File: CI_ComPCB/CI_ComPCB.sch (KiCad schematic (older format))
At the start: 9 parts, among them J101 Conn_01x15_Female, J102 Conn_01x15_Female, U101 ESP32s

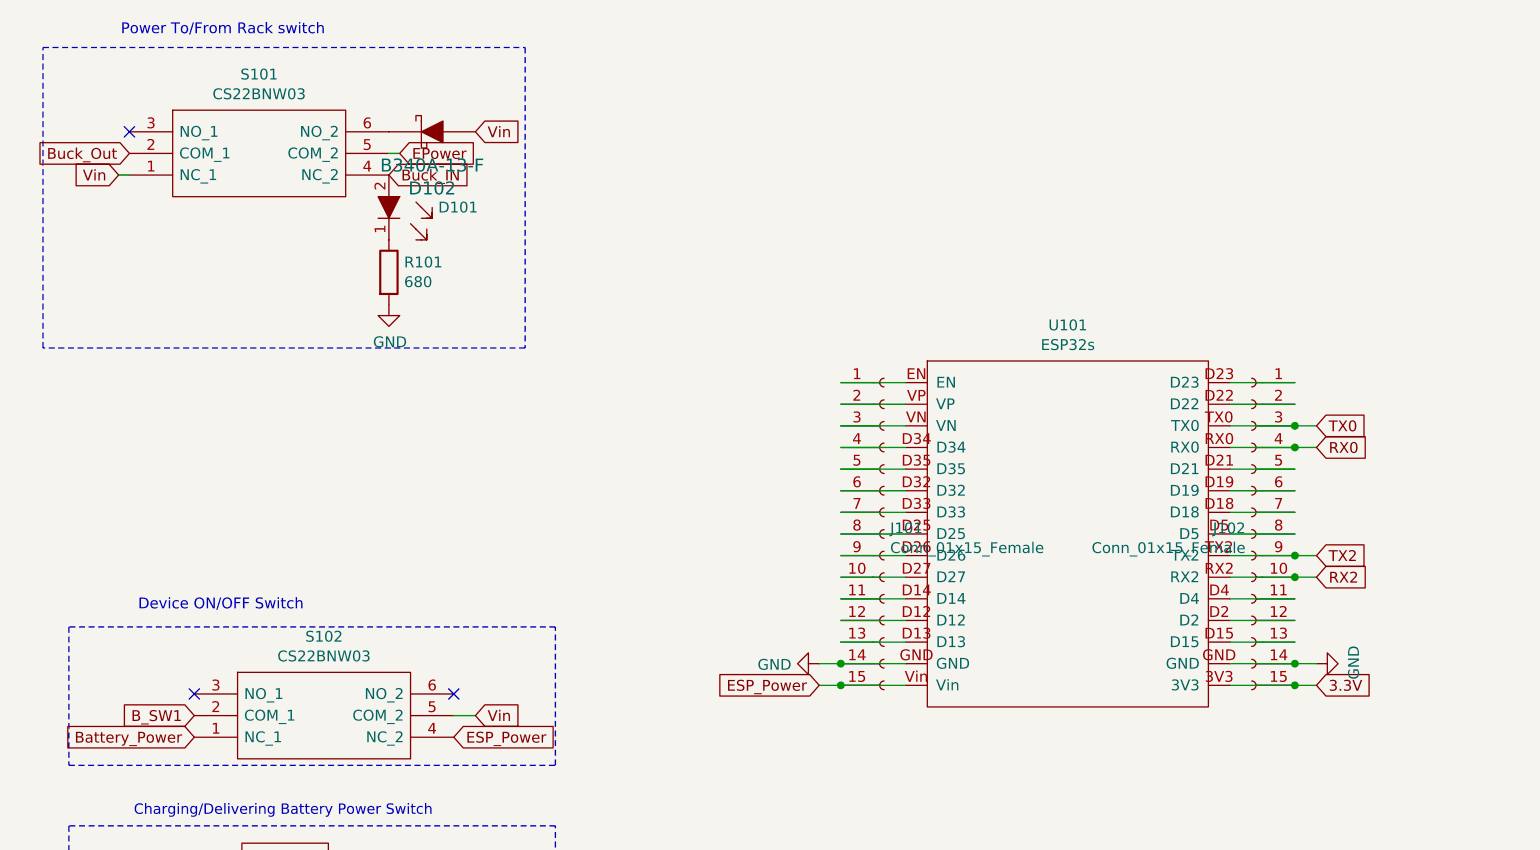
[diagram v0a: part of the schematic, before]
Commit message: V1.1 in progress
Completed Bom and schematic
still need to add routs and PCB layout
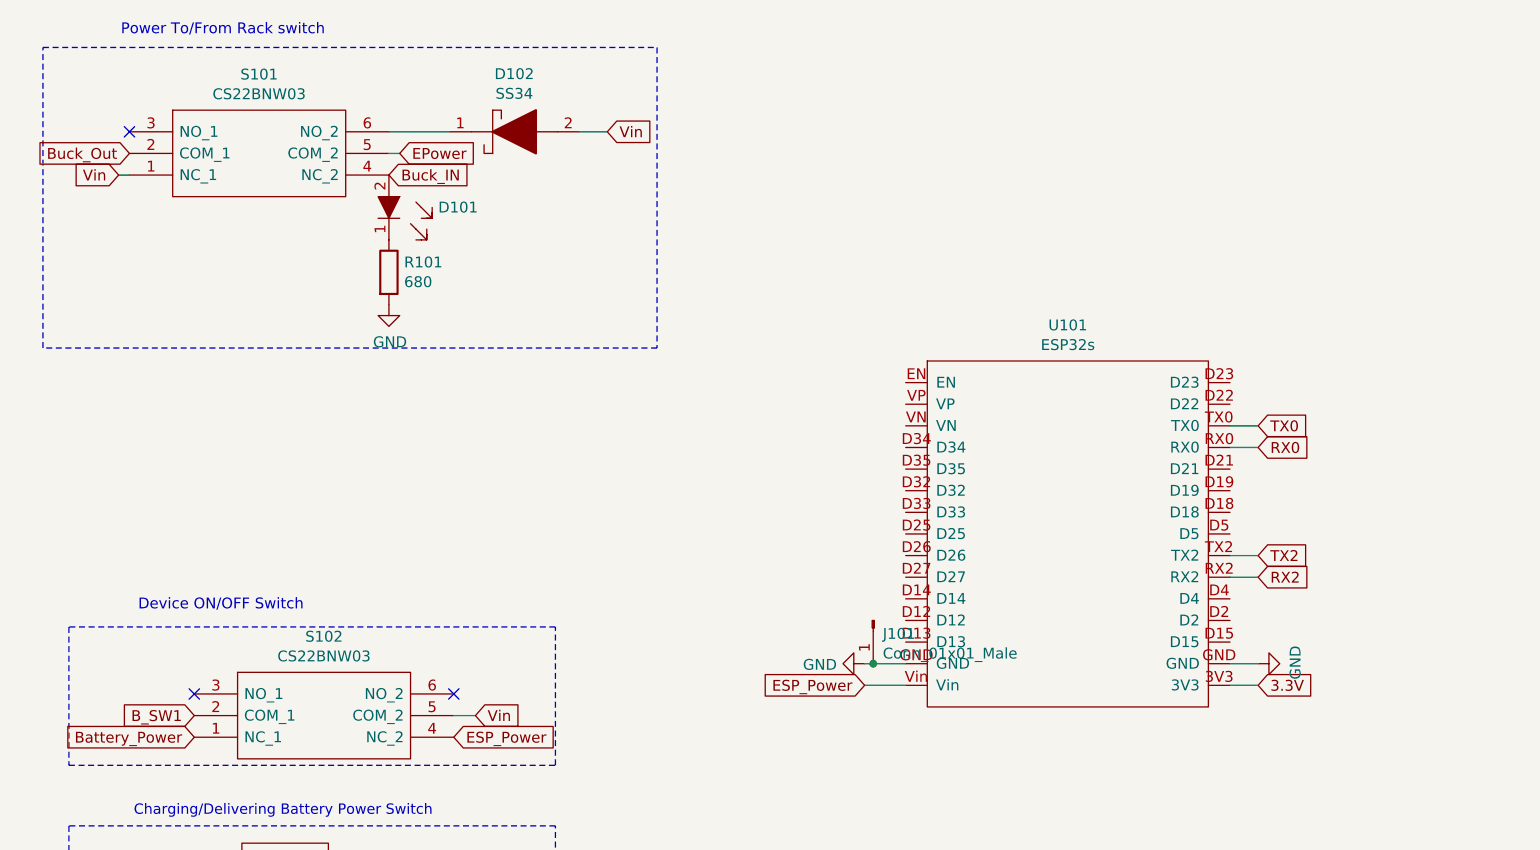
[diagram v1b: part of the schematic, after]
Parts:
- removed D102: B340A-13-F, digikey-footprints:DO-214AC, symbol dk_Diodes-Rectifiers-Single:B340A-13-F
- removed J101, J102: Conn_01x15_Female, Connector_PinSocket_2.54mm:PinSocket_1x15_P2.54mm_Vertical, symbol Connector:Conn_01x15_Female
- added D102: SS34, SamacSys_Parts:DIOM8059X256N, symbol SamacSys_Parts:SS34
- added J101: Conn_01x01_Male, Connector_PinHeader_2.54mm:PinHeader_1x01_P2.54mm_Vertical, symbol Connector:Conn_01x01_Male
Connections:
- net GND: now also J101.1 (Pin_1)
- net Vin: now also D102.2
- net at S101.6 (NO_2): now also D102.1
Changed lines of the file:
@@
 Comment4 ""
 $EndDescr
-Text GLabel 6750 3220 2    50   Input ~ 0
+Text GLabel 6480 3220 2    50   Input ~ 0
 RX0
-Text GLabel 6750 3120 2    50   Input ~ 0
+Text GLabel 6480 3120 2    50   Input ~ 0
 TX0
-Text GLabel 6750 3720 2    50   Input ~ 0
+Text GLabel 6480 3720 2    50   Input ~ 0
 TX2
-Text GLabel 6750 3820 2    50   Input ~ 0
+Text GLabel 6480 3820 2    50   Input ~ 0
 RX2
-Text GLabel 6750 4320 2    50   Input ~ 0
+Text GLabel 6480 4320 2    50   Input ~ 0
 3.3V
 $Comp
@@
 L power:GND #PWR0103
 U 1 1 6128A8B5
-P 6750 4220
-F 0 "#PWR0103" H 6750 3970 50  0001 C CNN
-F 1 "GND" H 6755 4047 50  0000 C CNN
-F 2 "" H 6750 4220 50  0001 C CNN
-F 3 "" H 6750 4220 50  0001 C CNN
-	1    6750 4220
+P 6480 4220
+F 0 "#PWR0103" H 6480 3970 50  0001 C CNN
+F 1 "GND" H 6485 4047 50  0000 C CNN
+F 2 "" H 6480 4220 50  0001 C CNN
+F 3 "" H 6480 4220 50  0001 C CNN
+	1    6480 4220
 	0    -1   -1   0
 $EndComp
@@
 L power:GND #PWR0102
 U 1 1 612B87BD
-P 4450 4220
-F 0 "#PWR0102" H 4450 3970 50  0001 C CNN
-F 1 "GND" V 4455 4092 50  0000 R CNN
-F 2 "" H 4450 4220 50  0001 C CNN
-F 3 "" H 4450 4220 50  0001 C CNN
-	1    4450 4220
+P 4660 4220
+F 0 "#PWR0102" H 4660 3970 50  0001 C CNN
+F 1 "GND" V 4665 4092 50  0000 R CNN
+F 2 "" H 4660 4220 50  0001 C CNN
+F 3 "" H 4660 4220 50  0001 C CNN
+	1    4660 4220
 	0    1    1    0
 $EndComp
@@
 Text Notes 1300 3980 0    50   ~ 0
 Device ON/OFF Switch
-Text GLabel 4450 4320 0    50   Input ~ 0
+Text GLabel 4660 4320 0    50   Input ~ 0
 ESP_Power
 Wire Wire Line
@@
 Text Notes 1220 1320 0    50   ~ 0
 Power To/From Rack switch
-Text GLabel 2860 1760 2    50   Input ~ 0
+Text GLabel 3470 1760 2    50   Input ~ 0
 Vin
 Wire Wire Line
@@
 $EndComp
 Wire Notes Line
-	3090 2760 860  2760
+	3700 2760 860  2760
 Wire Notes Line
 	860  2760 860  1370
 Wire Notes Line
-	860  1370 3090 1370
-Wire Notes Line
-	3090 1370 3090 2760
+	860  1370 3700 1370
+Wire Notes Line
+	3700 1370 3700 2760
 Wire Notes Line
 	980  4690 3230 4690
@@
 Wire Notes Line
 	980  4050 980  4690
-$Comp
-L dk_Diodes-Rectifiers-Single:B340A-13-F D102
-U 1 1 619E1DE9
-P 2660 1760
-F 0 "D102" H 2660 2022 60  0000 C CNN
-F 1 "B340A-13-F" H 2660 1916 60  0000 C CNN
-F 2 "digikey-footprints:DO-214AC" H 2860 1960 60  0001 L CNN
-F 3 "https://www.diodes.com/assets/Datasheets/ds30891.pdf" H 2860 2060 60  0001 L CNN
-F 4 "B340A-FDICT-ND" H 2860 2160 60  0001 L CNN "Digi-Key_PN"
-F 5 "B340A-13-F" H 2860 2260 60  0001 L CNN "MPN"
-F 6 "Discrete Semiconductor Products" H 2860 2360 60  0001 L CNN "Category"
-F 7 "Diodes - Rectifiers - Single" H 2860 2460 60  0001 L CNN "Family"
-F 8 "https://www.diodes.com/assets/Datasheets/ds30891.pdf" H 2860 2560 60  0001 L CNN "DK_Datasheet_Link"
-F 9 "/product-detail/en/diodes-incorporated/B340A-13-F/B340A-FDICT-ND/725054" H 2860 2660 60  0001 L CNN "DK_Detail_Page"
-F 10 "DIODE SCHOTTKY 40V 3A SMA" H 2860 2760 60  0001 L CNN "Description"
-F 11 "Diodes Incorporated" H 2860 2860 60  0001 L CNN "Manufacturer"
-F 12 "Active" H 2860 2960 60  0001 L CNN "Status"
-	1    2660 1760
-	-1   0    0    1
-$EndComp
 $Sheet
 S 8660 6040 2540 380
@@
 Charging/Delivering Battery Power Switch
 Wire Wire Line
-	4850 3320 4550 3320
-Wire Wire Line
-	4850 3420 4550 3420
-Wire Wire Line
-	4850 3520 4550 3520
-Wire Wire Line
-	4850 3620 4550 3620
-Wire Wire Line
-	4850 3720 4550 3720
-Wire Wire Line
-	4850 3820 4550 3820
-Wire Wire Line
-	4850 3920 4550 3920
-Wire Wire Line
-	4850 4020 4550 4020
-Wire Wire Line
-	4850 4120 4550 4120
-Wire Wire Line
-	6350 4120 6650 4120
-Wire Wire Line
-	6350 4020 6650 4020
-Wire Wire Line
-	6350 3920 6650 3920
-Wire Wire Line
-	6350 3020 6650 3020
-Wire Wire Line
-	6350 3620 6650 3620
-Wire Wire Line
-	6350 3520 6650 3520
-Wire Wire Line
-	6350 3420 6650 3420
-Wire Wire Line
-	6350 3320 6650 3320
-Wire Wire Line
-	6650 3720 6750 3720
-Wire Wire Line
-	6350 3720 6650 3720
-Connection ~ 6650 3720
-Wire Wire Line
-	6650 3220 6750 3220
-Wire Wire Line
-	6350 3220 6650 3220
-Connection ~ 6650 3220
-Wire Wire Line
-	6650 3120 6750 3120
-Wire Wire Line
-	6350 3120 6650 3120
-Connection ~ 6650 3120
-Wire Wire Line
-	6650 4320 6750 4320
-Wire Wire Line
-	6350 4320 6650 4320
-Connection ~ 6650 4320
-Wire Wire Line
-	6650 4220 6750 4220
-Wire Wire Line
-	6350 4220 6650 4220
-Connection ~ 6650 4220
-Wire Wire Line
-	6650 3820 6750 3820
-Wire Wire Line
-	6350 3820 6650 3820
-Connection ~ 6650 3820
-$Comp
-L Connector:Conn_01x15_Female J102
-U 1 1 6118396F
-P 6450 3620
-F 0 "J102" H 6478 3646 50  0000 L CNN
-F 1 "Conn_01x15_Female" H 6478 3555 50  0000 L CNN
-F 2 "Connector_PinSocket_2.54mm:PinSocket_1x15_P2.54mm_Vertical" H 6450 3620 50  0001 C CNN
-F 3 "~" H 6450 3620 50  0001 C CNN
-	1    6450 3620
-	-1   0    0    -1
-$EndComp
-Wire Wire Line
-	6350 2920 6650 2920
-Wire Wire Line
-	4850 2920 4550 2920
-Wire Wire Line
-	4850 3020 4550 3020
-Wire Wire Line
-	4850 3120 4550 3120
-Wire Wire Line
-	4850 3220 4550 3220
-Wire Wire Line
-	4550 4320 4450 4320
-Wire Wire Line
-	4850 4320 4550 4320
-Connection ~ 4550 4320
-Wire Wire Line
-	4850 4220 4550 4220
-Wire Wire Line
-	4550 4220 4450 4220
-Connection ~ 4550 4220
-$Comp
-L Connector:Conn_01x15_Female J101
-U 1 1 6118647F
-P 4750 3620
-F 0 "J101" H 4778 3646 50  0000 L CNN
-F 1 "Conn_01x15_Female" H 4778 3555 50  0000 L CNN
-F 2 "Connector_PinSocket_2.54mm:PinSocket_1x15_P2.54mm_Vertical" H 4750 3620 50  0001 C CNN
-F 3 "~" H 4750 3620 50  0001 C CNN
-	1    4750 3620
-	1    0    0    -1
-$EndComp
+	4660 4220 4700 4220
+Wire Wire Line
+	4660 4320 4850 4320
+Wire Wire Line
+	6350 3820 6480 3820
+Wire Wire Line
+	6350 4220 6480 4220
+Wire Wire Line
+	6350 4320 6480 4320
+Wire Wire Line
+	6350 3120 6480 3120
+Wire Wire Line
+	6350 3220 6480 3220
+Wire Wire Line
+	6350 3720 6480 3720
+$Comp
+L Connector:Conn_01x01_Male J101
+U 1 1 61290C13
+P 4700 4020
+F 0 "J101" V 4762 4064 50  0000 L CNN
+F 1 "Conn_01x01_Male" V 4853 4064 50  0000 L CNN
+F 2 "Connector_PinHeader_2.54mm:PinHeader_1x01_P2.54mm_Vertical" H 4700 4020 50  0001 C CNN
+F 3 "~" H 4700 4020 50  0001 C CNN
+	1    4700 4020
+	0    1    1    0
+$EndComp
+Connection ~ 4700 4220
+Wire Wire Line
+	4700 4220 4850 4220
+$Comp
+L SamacSys_Parts:SS34 D102
+U 1 1 612A21DD
+P 2640 1760
+F 0 "D102" H 3040 2027 50  0000 C CNN
+F 1 "SS34" H 3040 1936 50  0000 C CNN
+F 2 "SamacSys_Parts:DIOM8059X256N" H 3140 1910 50  0001 L CNN
+F 3 "https://componentsearchengine.com/Datasheets/2/SS34.pdf" H 3140 1810 50  0001 L CNN
+F 4 "ON Semi SS34 SMT Schottky Diode, 40V 3A, 2-Pin DO-214AB" H 3140 1710 50  0001 L CNN "Description"
+F 5 "2.56" H 3140 1610 50  0001 L CNN "Height"
+F 6 "512-SS34" H 3140 1510 50  0001 L CNN "Mouser Part Number"
+F 7 "https://www.mouser.co.uk/ProductDetail/ON-Semiconductor-Fairchild/SS34?qs=2ONuHmP%2FXzb3ub11UdFfdQ%3D%3D" H 3140 1410 50  0001 L CNN "Mouser Price/Stock"
+F 8 "ON Semiconductor" H 3140 1310 50  0001 L CNN "Manufacturer_Name"
+F 9 "SS34" H 3140 1210 50  0001 L CNN "Manufacturer_Part_Number"
+	1    2640 1760
+	1    0    0    -1
+$EndComp
+Wire Wire Line
+	2460 1760 2740 1760
+Wire Wire Line
+	3470 1760 3340 1760
 $EndSCHEMATC

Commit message: V1.1 Rough
Almost complete
needs silk screen annotations then will be ready to have printed
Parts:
- added H101, H102, H103, H104: MountingHole_Pad, MountingHole:MountingHole_3.2mm_M3_ISO7380_Pad_TopBottom, symbol Mechanical:MountingHole_Pad
- D101: symbol dk_LED-Indication-Discrete:LTST-C190GKT -> CI_ComPCB-rescue:LTST-C190GKT-dk_LED-Indication-Discrete
- D102: symbol SamacSys_Parts:SS34 -> CI_ComPCB-rescue:SS34-SamacSys_Parts
- S101, S102: symbol SamacSys_Parts:CS22BNW03 -> CI_ComPCB-rescue:CS22BNW03-SamacSys_Parts
- S103: symbol SamacSys_Parts:CS12ANW03 -> CI_ComPCB-rescue:CS12ANW03-SamacSys_Parts
- U101: symbol CI_ComPCB-rescue:ESP32s-RackComm-rescue -> CI_ComPCB-rescue:ESP32s-RackComm-rescue-CI_ComPCB-rescue
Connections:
- net GND: now also H101.1, H102.1, H103.1, H104.1
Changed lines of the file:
@@
 3.3V
 $Comp
-L CI_ComPCB-rescue:ESP32s-RackComm-rescue U101
+L CI_ComPCB-rescue:ESP32s-RackComm-rescue-CI_ComPCB-rescue U101
 U 1 1 61536F0E
 P 4750 2820
@@
 Buck_Out
 $Comp
-L SamacSys_Parts:CS22BNW03 S102
+L CI_ComPCB-rescue:CS22BNW03-SamacSys_Parts S102
 U 1 1 61678194
 P 1560 4360
@@
 $EndComp
 $Comp
-L SamacSys_Parts:CS22BNW03 S101
+L CI_ComPCB-rescue:CS22BNW03-SamacSys_Parts S101
 U 1 1 6172901A
 P 1260 1760
@@
 $EndComp
 $Comp
-L dk_LED-Indication-Discrete:LTST-C190GKT D101
+L CI_ComPCB-rescue:LTST-C190GKT-dk_LED-Indication-Discrete D101
 U 1 1 6128530A
 P 2460 2160
@@
 Vin
 $Comp
-L SamacSys_Parts:CS12ANW03 S103
+L CI_ComPCB-rescue:CS12ANW03-SamacSys_Parts S103
 U 1 1 61AC507A
 P 2380 5350
@@
 	4700 4220 4850 4220
 $Comp
-L SamacSys_Parts:SS34 D102
+L CI_ComPCB-rescue:SS34-SamacSys_Parts D102
 U 1 1 612A21DD
 P 2640 1760
@@
 Wire Wire Line
 	3470 1760 3340 1760
+$Comp
+L Mechanical:MountingHole_Pad H102
+U 1 1 612ABAC3
+P 9900 3550
+F 0 "H102" H 10000 3599 50  0000 L CNN
+F 1 "MountingHole_Pad" H 10000 3508 50  0000 L CNN
+F 2 "MountingHole:MountingHole_3.2mm_M3_ISO7380_Pad_TopBottom" H 9900 3550 50  0001 C CNN
+F 3 "~" H 9900 3550 50  0001 C CNN
+	1    9900 3550
+	1    0    0    -1
+$EndComp
+$Comp
+L Mechanical:MountingHole_Pad H104
+U 1 1 612ABFD3
+P 10250 3550
+F 0 "H104" H 10350 3599 50  0000 L CNN
+F 1 "MountingHole_Pad" H 10350 3508 50  0000 L CNN
+F 2 "MountingHole:MountingHole_3.2mm_M3_ISO7380_Pad_TopBottom" H 10250 3550 50  0001 C CNN
+F 3 "~" H 10250 3550 50  0001 C CNN
+	1    10250 3550
+	1    0    0    -1
+$EndComp
+$Comp
+L Mechanical:MountingHole_Pad H101
+U 1 1 612AC52F
+P 9900 3300
+F 0 "H101" H 10000 3349 50  0000 L CNN
+F 1 "MountingHole_Pad" H 10000 3258 50  0000 L CNN
+F 2 "MountingHole:MountingHole_3.2mm_M3_ISO7380_Pad_TopBottom" H 9900 3300 50  0001 C CNN
+F 3 "~" H 9900 3300 50  0001 C CNN
+	1    9900 3300
+	1    0    0    -1
+$EndComp
+$Comp
+L Mechanical:MountingHole_Pad H103
+U 1 1 612ACC04
+P 10250 3300
+F 0 "H103" H 10350 3349 50  0000 L CNN
+F 1 "MountingHole_Pad" H 10350 3258 50  0000 L CNN
+F 2 "MountingHole:MountingHole_3.2mm_M3_ISO7380_Pad_TopBottom" H 10250 3300 50  0001 C CNN
+F 3 "~" H 10250 3300 50  0001 C CNN
+	1    10250 3300
+	1    0    0    -1
+$EndComp
+Wire Wire Line
+	9900 3650 10100 3650
+Wire Wire Line
+	10250 3650 10250 3400
+Connection ~ 10250 3650
+Wire Wire Line
+	10250 3400 9900 3400
+Connection ~ 10250 3400
+Wire Wire Line
+	9900 3400 9900 3650
+Connection ~ 9900 3400
+Connection ~ 9900 3650
+$Comp
+L power:GND #PWR0104
+U 1 1 612AE626
+P 10100 3650
+F 0 "#PWR0104" H 10100 3400 50  0001 C CNN
+F 1 "GND" H 10105 3477 50  0000 C CNN
+F 2 "" H 10100 3650 50  0001 C CNN
+F 3 "" H 10100 3650 50  0001 C CNN
+	1    10100 3650
+	1    0    0    -1
+$EndComp
+Connection ~ 10100 3650
+Wire Wire Line
+	10100 3650 10250 3650
 $EndSCHEMATC

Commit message: V1.1 Changed Diode for reprint
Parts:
- D102: footprint SamacSys_Parts:DIOM8059X256N -> digikey-footprints:DO-214AC
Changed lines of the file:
@@
 F 0 "D102" H 3040 2027 50  0000 C CNN
 F 1 "SS34" H 3040 1936 50  0000 C CNN
-F 2 "SamacSys_Parts:DIOM8059X256N" H 3140 1910 50  0001 L CNN
+F 2 "digikey-footprints:DO-214AC" H 3140 1910 50  0001 L CNN
 F 3 "https://componentsearchengine.com/Datasheets/2/SS34.pdf" H 3140 1810 50  0001 L CNN
 F 4 "ON Semi SS34 SMT Schottky Diode, 40V 3A, 2-Pin DO-214AB" H 3140 1710 50  0001 L CNN "Description"

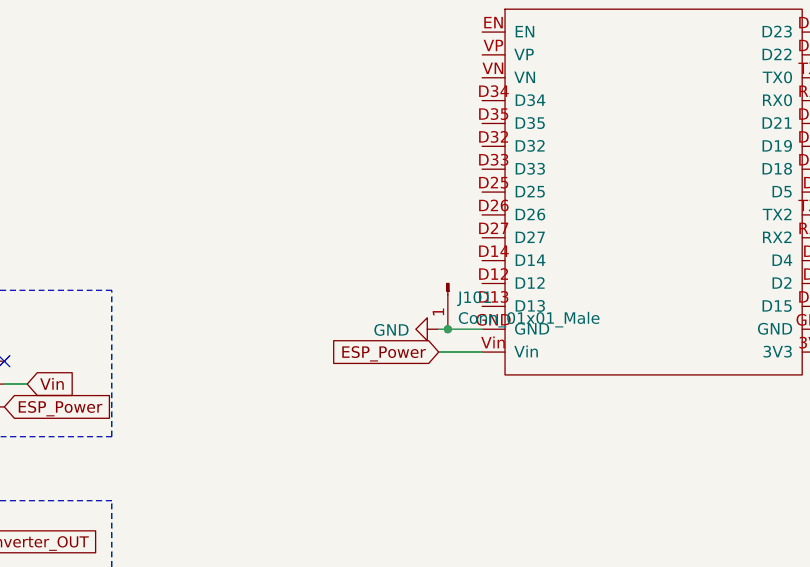
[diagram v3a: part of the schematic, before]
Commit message: switch
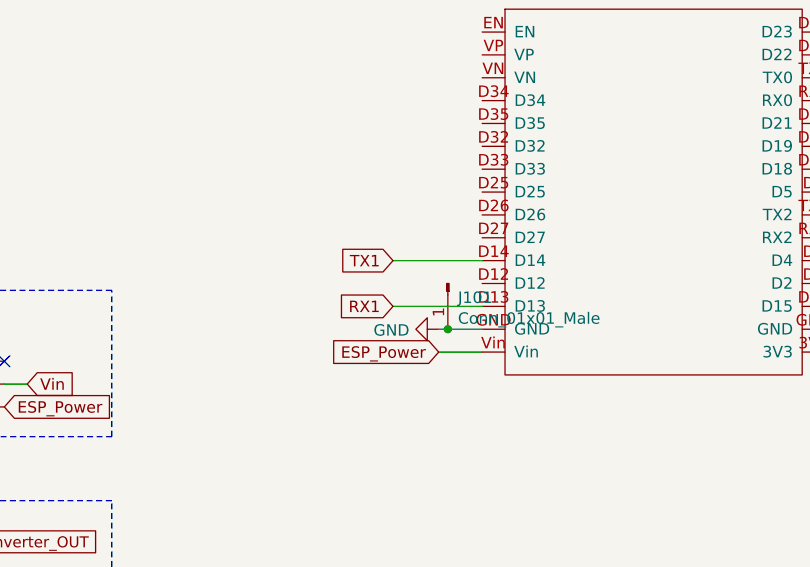
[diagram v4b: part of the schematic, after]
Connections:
- net RX1: now reaches U101.D13
- net TX1: now reaches U101.D14
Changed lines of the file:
@@
 Wire Wire Line
 	10100 3650 10250 3650
+Wire Wire Line
+	4850 4120 4460 4120
+Wire Wire Line
+	4850 3920 4460 3920
+Text GLabel 4460 4120 0    50   Input ~ 0
+RX1
+Text GLabel 4460 3920 0    50   Input ~ 0
+TX1
 $EndSCHEMATC
